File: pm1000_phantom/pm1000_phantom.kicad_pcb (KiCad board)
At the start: 2 copper layers, 27 x 44.5 mm, 17 parts, among them J1 2 pin 2,54mm Molex, J10 2 pin 2,54mm Molex, J2 2 pin 2,54mm Molex, J3 2 pin 2,54mm Molex, J4 2 pin 2,54mm Molex, J5 2 pin 2,54mm Molex, J6 3 pin 2,54mm Molex, J7 3 pin 2,54mm Molex, J8 3 pin 2,54mm Molex, J9 3 pin 2,54mm Molex

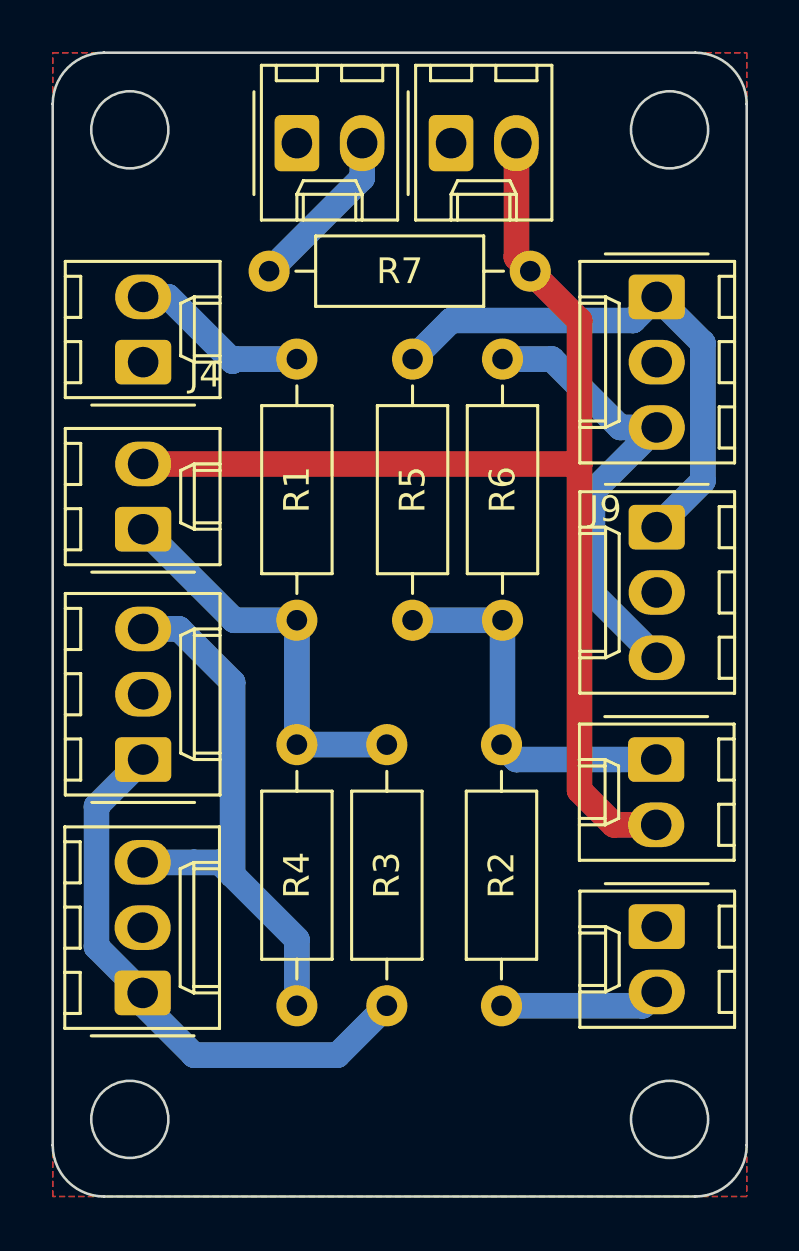
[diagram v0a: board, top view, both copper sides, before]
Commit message: fix phantom board labels
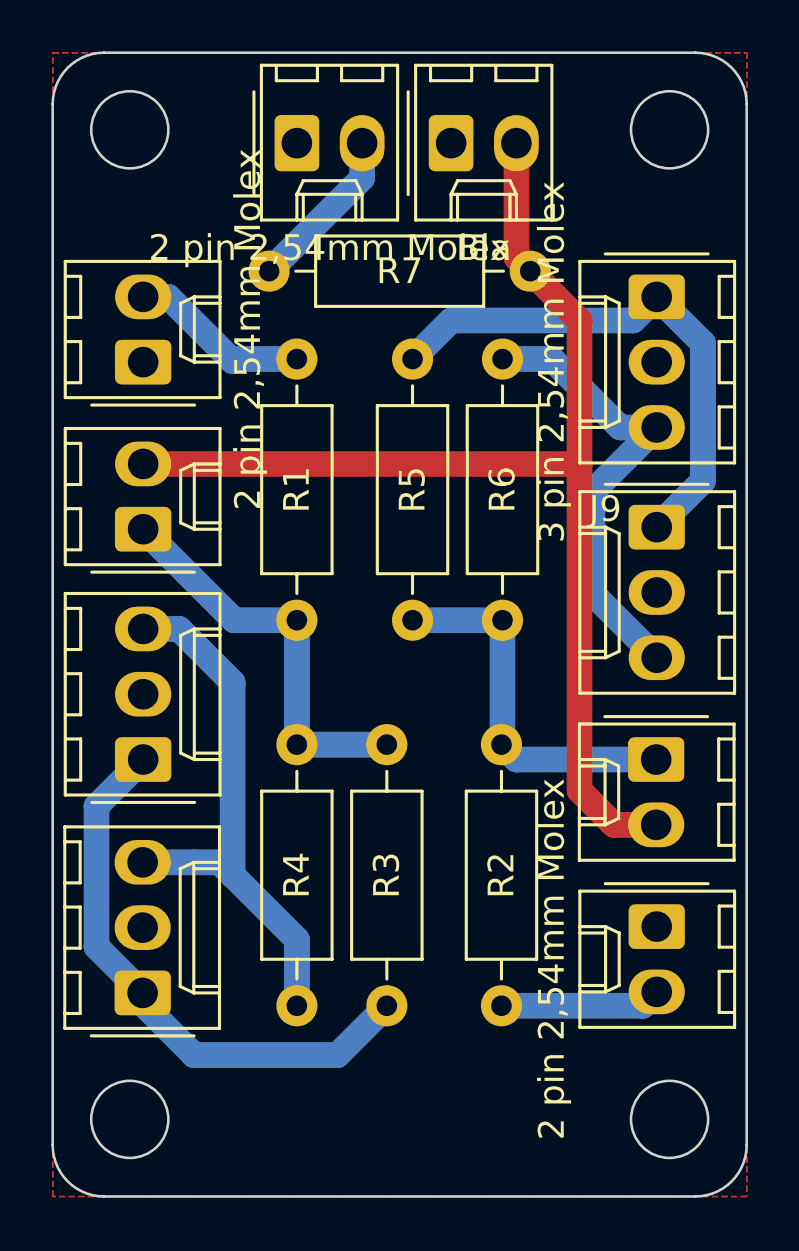
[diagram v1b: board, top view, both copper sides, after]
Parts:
- J1: value 2 pin 2,54mm Molex -> Bla
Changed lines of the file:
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@@
 		(property "Value" "3 pin 2,54mm Molex"
 			(at 2.54 4.08 90)
-			(layer "F.Fab")
-			(hide yes)
+			(layer "F.SilkS")
 			(effects
 				(font
@@
 		(property "Value" "2 pin 2,54mm Molex"
 			(at 1.27 4.08 0)
-			(layer "F.Fab")
-			(hide yes)
+			(layer "F.SilkS")
 			(effects
 				(font
@@
 			)
 		)
-		(property "Value" "2 pin 2,54mm Molex"
+		(property "Value" "Bla"
 			(at 1.27 4.08 0)
-			(layer "F.Fab")
-			(hide yes)
+			(layer "F.SilkS")
 			(effects
 				(font
@@
 			(at -2.54 3.81 0)
 			(layer "F.Fab")
-			(hide yes)
 			(effects
 				(font
@@
 			(at -0.485 2.41 0)
 			(layer "F.SilkS")
+			(hide yes)
 			(effects
 				(font
@@
 		(property "Value" "2 pin 2,54mm Molex"
 			(at 1.27 4.08 90)
-			(layer "F.Fab")
+			(layer "F.SilkS")
 			(effects
 				(font
@@
 		(property "Value" "2 pin 2,54mm Molex"
 			(at 1.27 4.08 90)
-			(layer "F.Fab")
-			(hide yes)
+			(layer "F.SilkS")
 			(effects
 				(font
